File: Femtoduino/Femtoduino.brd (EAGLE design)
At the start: 30.1 x 47 mm, 17 parts, among them SW1 SWITCH, U1 MIC5205, U2 ATMEGA328P-AU, Y1 16MHz

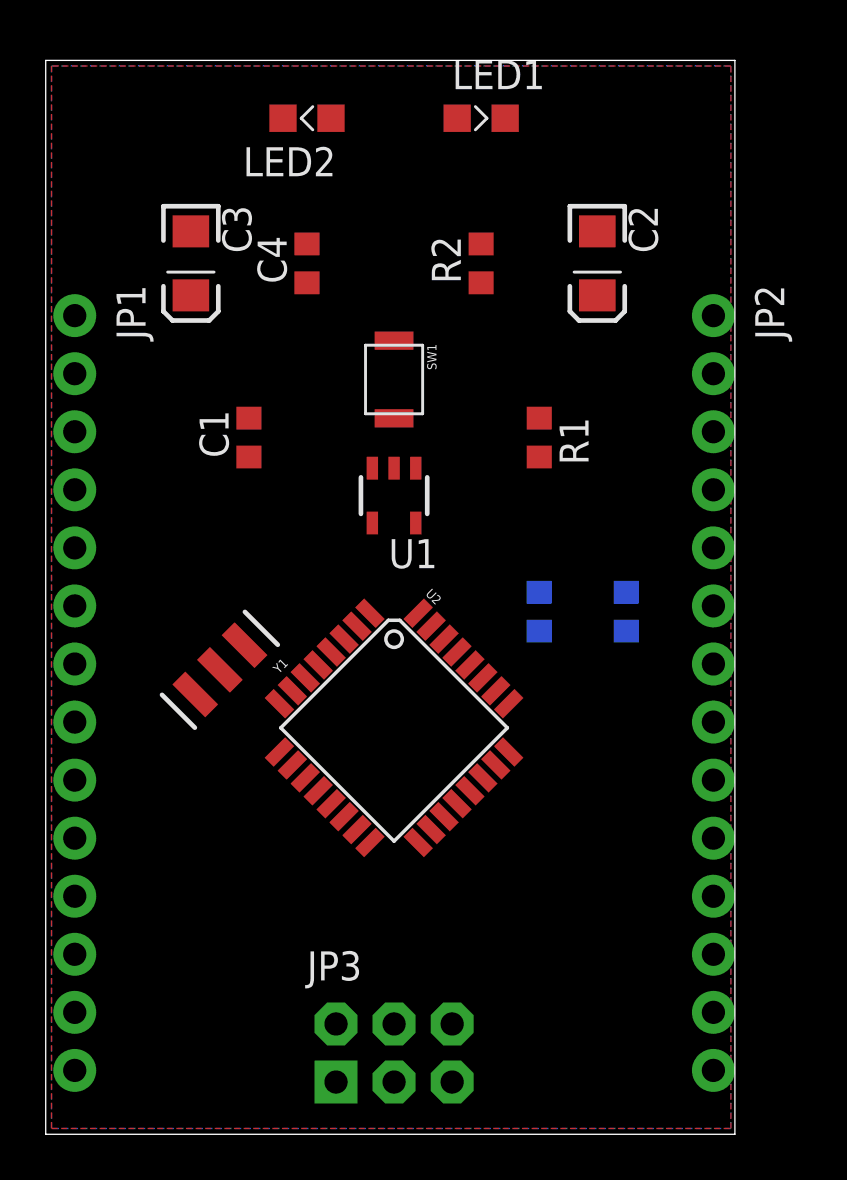
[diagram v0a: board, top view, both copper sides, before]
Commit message: Finished the routing and fill for the board
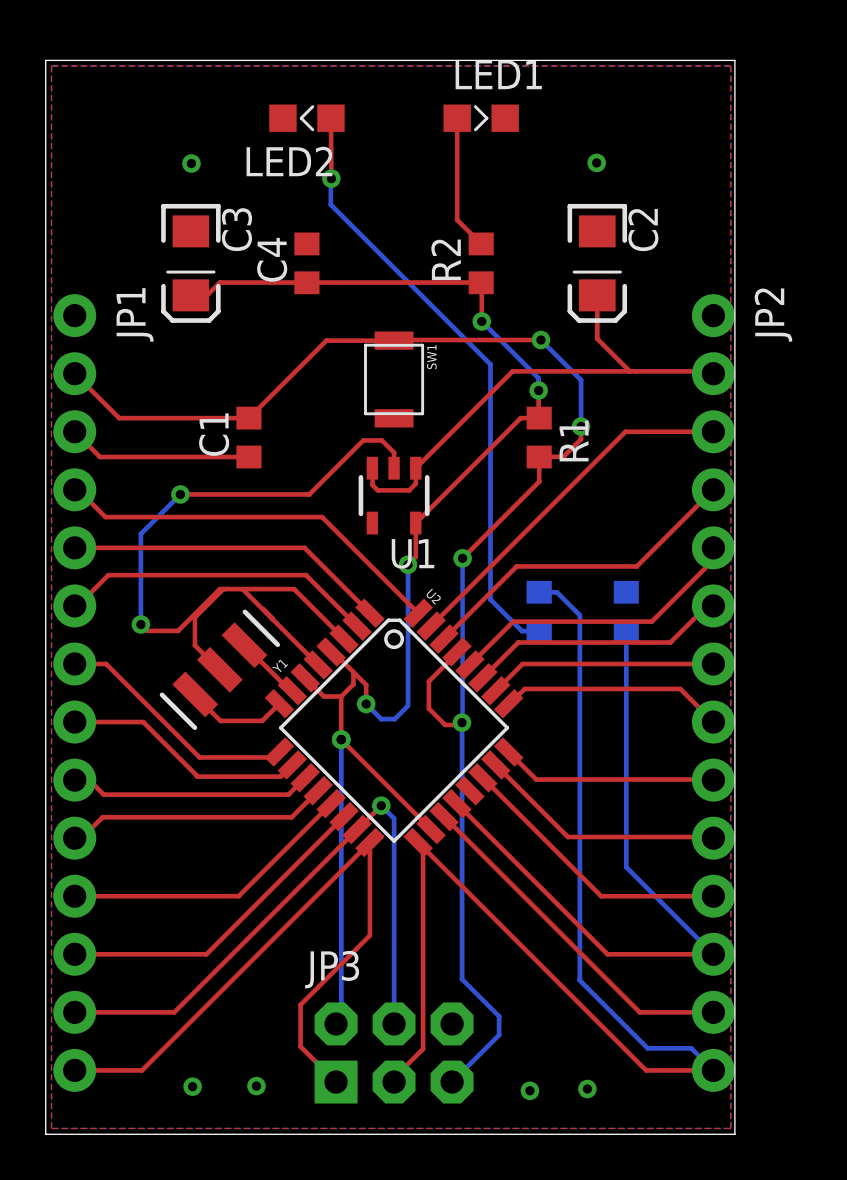
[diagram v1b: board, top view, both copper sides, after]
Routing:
- net RESET_N: track 0.00 -> 64.9 mm, vias 0 -> 4
- net VCC: track 0.00 -> 63.9 mm, vias 0 -> 6
- net D13/SCK: track 0.00 -> 53.8 mm
- net GND: track 0.00 -> 38.1 mm, vias 0 -> 8
- net AREF: track 0.00 -> 29.7 mm
- net D12/MISO: track 0.00 -> 29.4 mm
- net D11/MOSI: track 0.00 -> 26.9 mm, vias 0 -> 1
- net N$1: track 0.00 -> 26.7 mm, vias 0 -> 1
- net VIN: track 0.00 -> 22.3 mm
- net D2: track 0.00 -> 17.3 mm
- net D1: track 0.00 -> 15.9 mm
- net A6: track 0.00 -> 15.3 mm
- net D0: track 0.00 -> 14.5 mm
- net D10: track 0.00 -> 14.3 mm
- net D3: track 0.00 -> 14.1 mm
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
